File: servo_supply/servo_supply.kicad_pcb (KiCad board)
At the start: 2 copper layers, 46.3 x 37.8 mm, 26 parts, among them J1 Conn_01x02_Pin, J2 Conn_01x02_Pin, J3 Conn_01x02_Pin, U1 AZ1117-ADJ, U2 AZ1117-ADJ, U3 AZ1117-ADJ

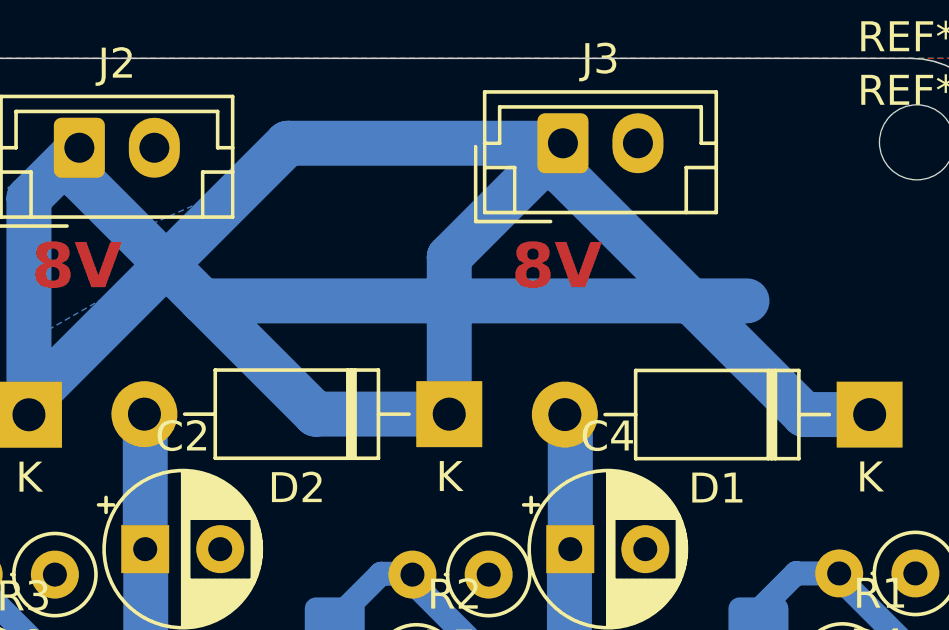
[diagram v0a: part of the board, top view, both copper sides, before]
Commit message: feat:bug修正
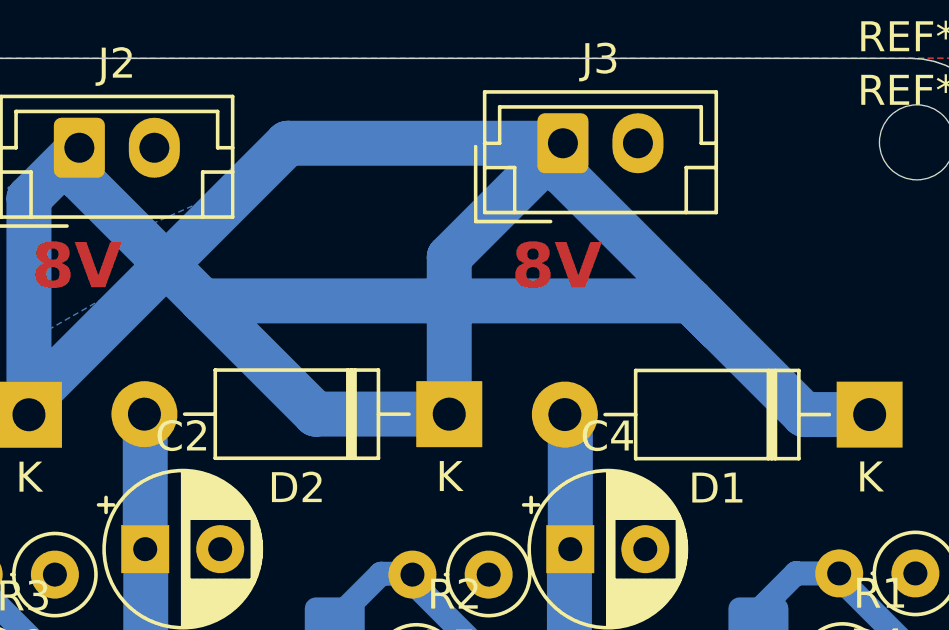
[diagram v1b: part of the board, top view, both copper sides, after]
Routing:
- net +8V: track 91.3 -> 90.7 mm
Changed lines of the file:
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@@
 	)
 	(segment
-		(start 175.235 80.285)
+		(start 174.295 81.225)
+		(end 173.355 80.285)
+		(width 1.5)
+		(layer "B.Cu")
+		(net 9)
+	)
+	(segment
+		(start 173.355 80.285)
 		(end 157.085 80.285)
 		(width 1.5)
